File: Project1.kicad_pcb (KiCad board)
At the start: 2 copper layers, 18.3 x 13.7 mm, 16 parts, among them J1 48037-0001, U1 MCP1702T-3302E/CB, U2 MCP6022T-I/ST

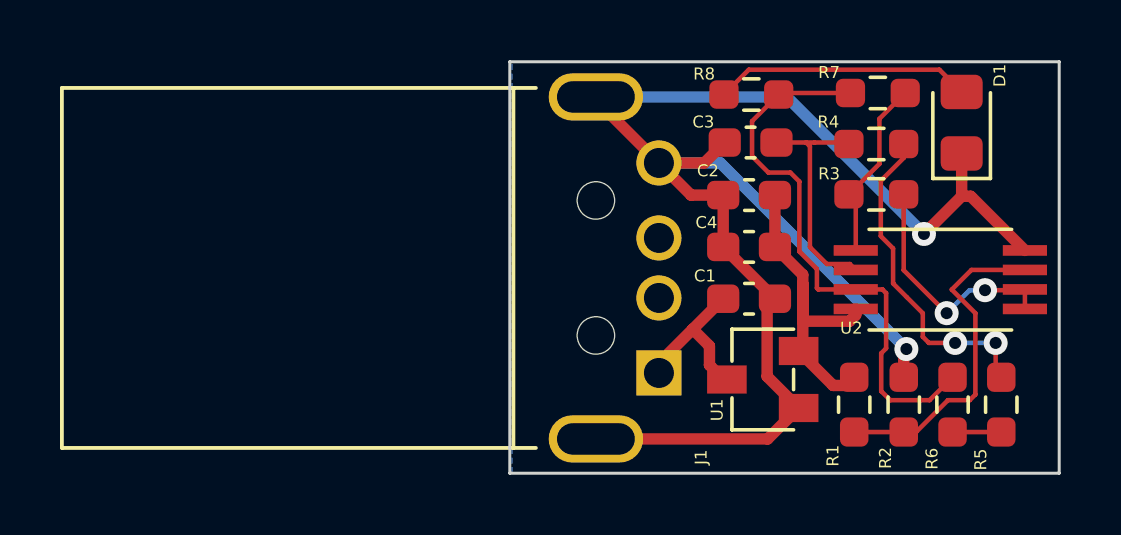
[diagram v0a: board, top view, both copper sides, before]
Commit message: Add report and necessary files
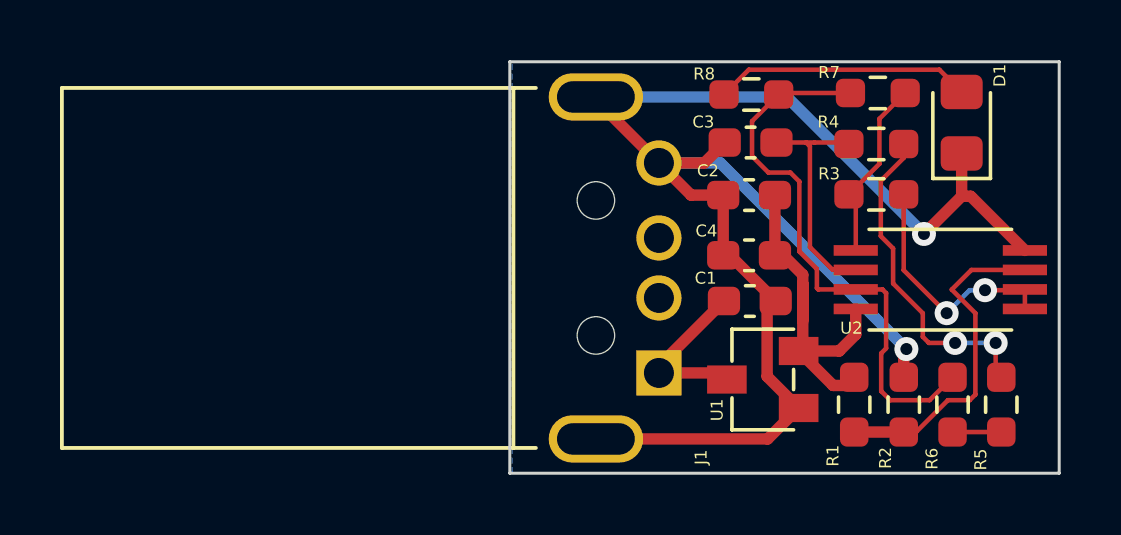
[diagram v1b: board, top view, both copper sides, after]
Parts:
- moved C4 0.28 mm to (36.0, 20.8)
- moved C1 0.08 mm to (36.0, 22.3)
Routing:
- net /VOUT_REG: track 11.5 -> 12.6 mm
- net /PWR_USB: track 5.54 -> 6.09 mm
